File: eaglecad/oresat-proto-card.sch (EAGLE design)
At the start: 263 parts, among them J6 J-SAMTEC-TFM-120-X1-XXX-D-RA, Q10 DMP2240UDM, Q11 MOSFET-PCH-SOT23-6, Q12 MOSFET-PCH-SOT23-6, Q13 PMV45EN, Q14 PMV45EN, Q15 DMP2240UDM, Q16 MOSFET-PCH-SOT23-6, Q17 MOSFET-PCH-SOT23-6, Q18 PMV45EN, Q19 PMV45EN, Q20 DMP2240UDM, Q21 MOSFET-PCH-SOT23-6, Q22 MOSFET-PCH-SOT23-6, Q23 PMV45EN, Q24 PMV45EN, Q25 DMP2240UDM, Q6 MOSFET-PCH-SOT23-6, Q7 MOSFET-PCH-SOT23-6, Q8 PMV45EN, Q9 PMV45EN, U10 MAX7310ATE, U11 MAX4211CETE, U12 MCP1703A, U13 MAX7310ATE, U14 MAX4211CETE, U15 MCP1703A, U3 MAX7310ATE, U4 MAX4211CETE, U6 MCP1703A, U7 MAX7310ATE, U8 MAX4211CETE, U9 MCP1703A

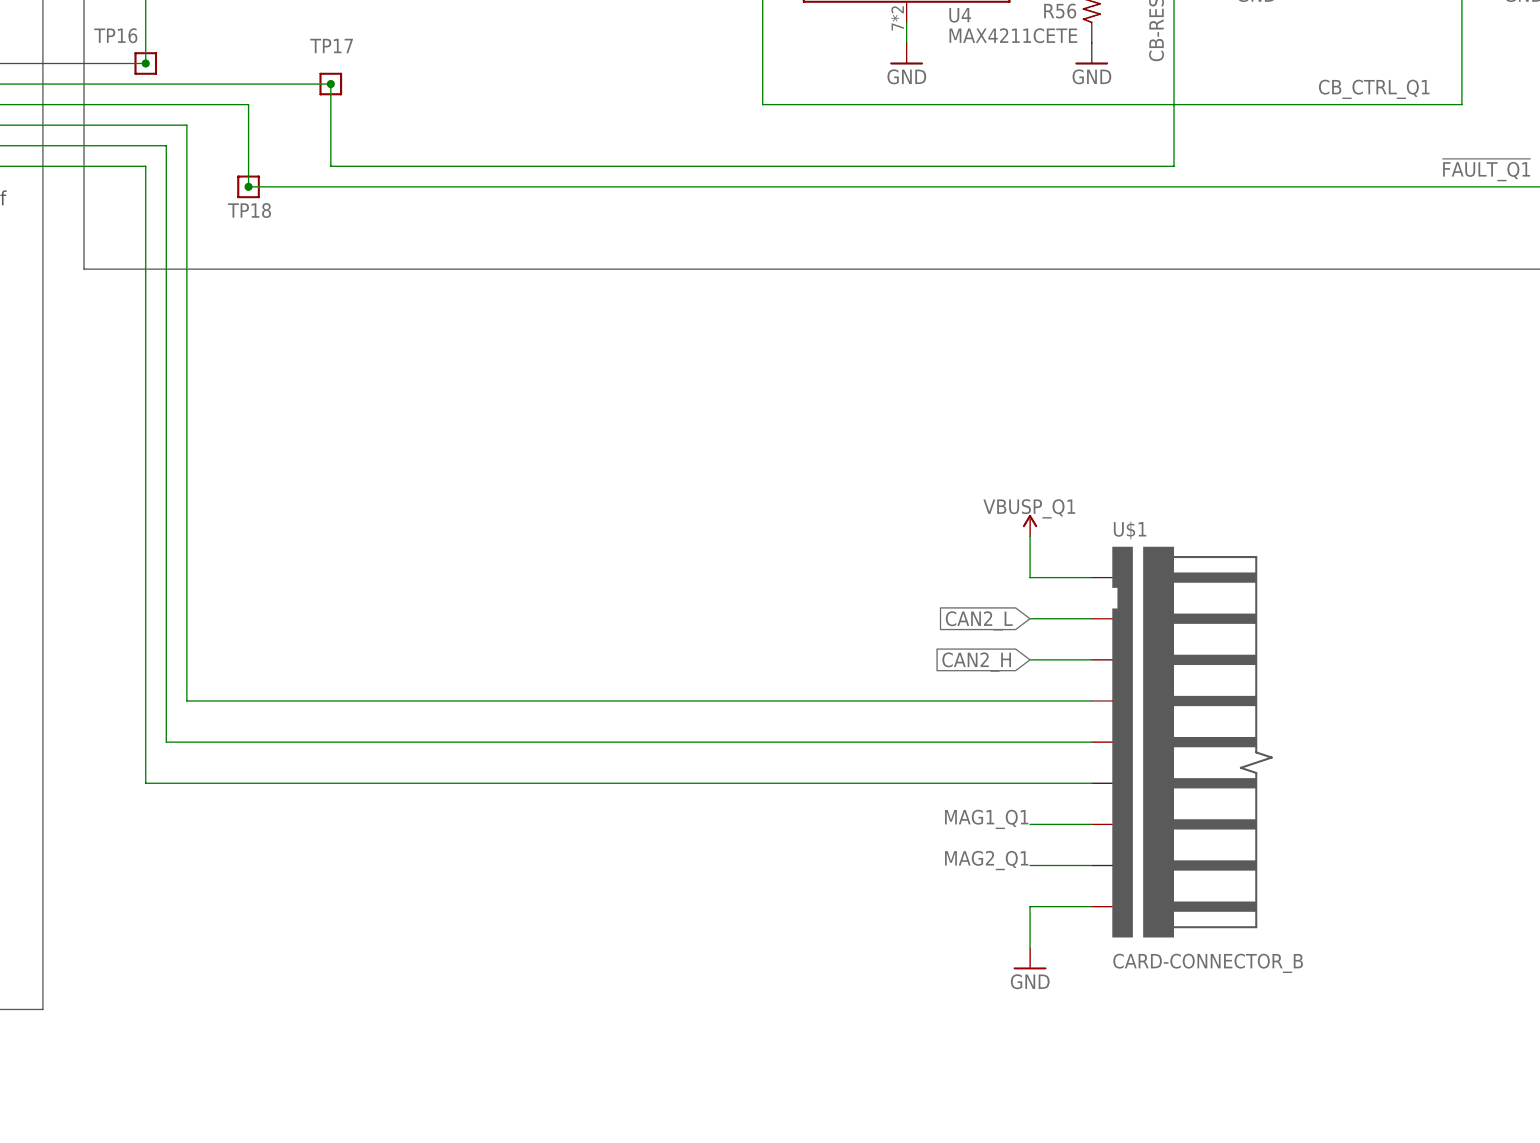
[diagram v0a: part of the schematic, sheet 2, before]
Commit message: card update
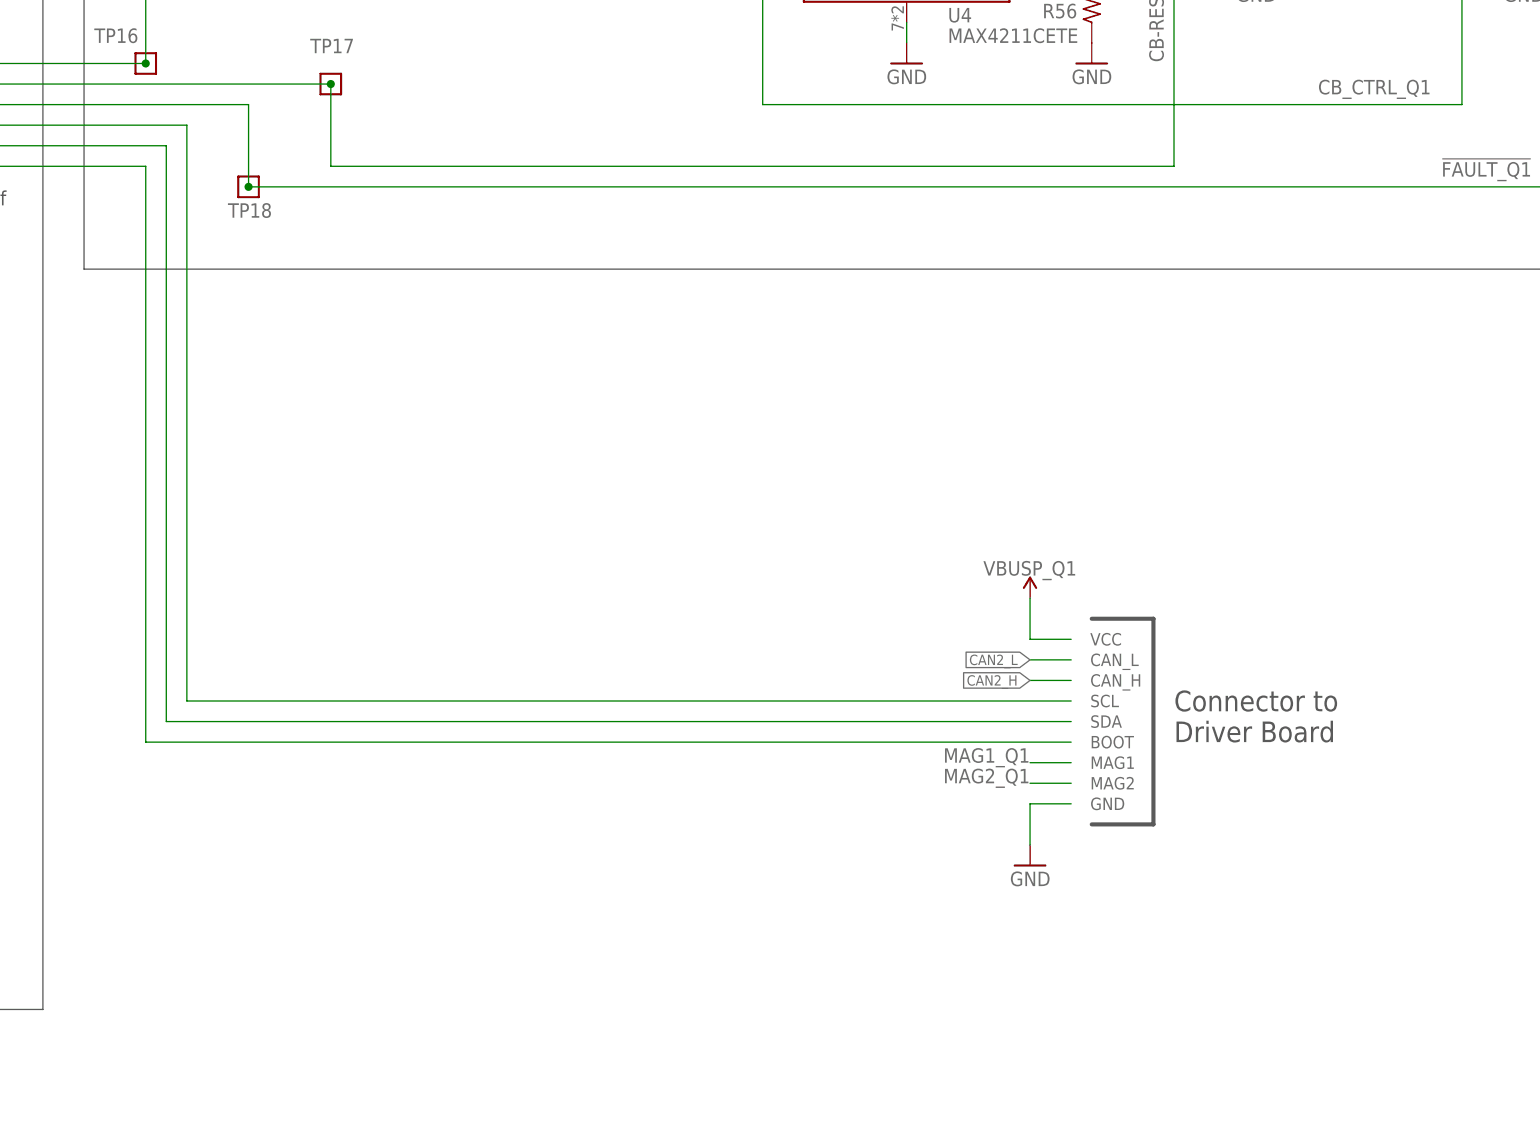
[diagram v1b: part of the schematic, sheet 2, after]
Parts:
- U$1: value CARD-CONNECTOR_B -> CARD-FLEX_CONNCARD-FLEX_CONN; device oresat-ACS_driver_board:CARD-CONNECTOR_B -> oresat-ACS_driver_board:CARD-FLEX_CONNCARD-FLEX_CONN
- U$3, U$4, U$5: value CARD-CONNECTOR_C -> CARD-FLEX_CONNCARD-FLEX_CONN; device oresat-ACS_driver_board:CARD-CONNECTOR_C -> oresat-ACS_driver_board:CARD-FLEX_CONNCARD-FLEX_CONN
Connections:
- net BOOT_Q1: now also U$3.BOOT; no longer U$1.P$6
- net BOOT_Q2: now also U$1.BOOT; no longer U$3.P$6
- net BOOT_Q3: now also U$4.BOOT; no longer U$4.P$6
- net BOOT_Q4: now also U$5.BOOT; no longer U$5.P$6
- net CAN2_H: now also U$1.CAN_H, U$3.CAN_H, U$4.CAN_H, U$5.CAN_H; no longer U$1.P$3, U$3.P$3, U$4.P$3, U$5.P$3
- net CAN2_L: now also U$1.CAN_L, U$3.CAN_L, U$4.CAN_L, U$5.CAN_L; no longer U$1.P$2, U$3.P$2, U$4.P$2, U$5.P$2
- net GND: now also U$1.GND, U$3.GND, U$4.GND, U$5.GND; no longer U$1.P$9, U$3.P$9, U$4.P$9, U$5.P$9
- net MAG1_Q1: now also U$3.MAG1; no longer U$1.P$7
- net MAG1_Q2: now also U$1.MAG1; no longer U$3.P$7
- net MAG1_Q3: now also U$4.MAG1; no longer U$4.P$7
- net MAG1_Q4: now also U$5.MAG1; no longer U$5.P$7
- net MAG2_Q1: now also U$3.MAG2; no longer U$1.P$8
- net MAG2_Q2: now also U$1.MAG2; no longer U$3.P$8
- net MAG2_Q3: now also U$4.MAG2; no longer U$4.P$8
- net MAG2_Q4: now also U$5.MAG2; no longer U$5.P$8
- net SCL_Q1: now also U$3.SCL; no longer U$1.P$4
- net SCL_Q2: now also U$1.SCL; no longer U$3.P$4
- net SCL_Q3: now also U$4.SCL; no longer U$4.P$4
- net SCL_Q4: now also U$5.SCL; no longer U$5.P$4
- net SDA_Q1: now also U$3.SDA; no longer U$1.P$5
- net SDA_Q2: now also U$1.SDA; no longer U$3.P$5
- net SDA_Q3: now also U$4.SDA; no longer U$4.P$5
- net SDA_Q4: now also U$5.SDA; no longer U$5.P$5
- net VBUSP_Q1: now also U$3.VCC; no longer U$1.P$1
- net VBUSP_Q2: now also U$1.VCC; no longer U$3.P$1
- net VBUSP_Q3: now also U$4.VCC; no longer U$4.P$1
- net VBUSP_Q4: now also U$5.VCC; no longer U$5.P$1
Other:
- note added: "Connector to Driver Board"
